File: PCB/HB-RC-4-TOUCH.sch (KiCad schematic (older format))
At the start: 13 parts, among them J1 Pad1, J2 Pad2, J3 Pad3, J4 Pad4, J5 SCL, J6 SDA, SW1 Config, U1 CC1101, U2 MPR121_Module-Touchpad, X1 Arduino_Pro_Mini

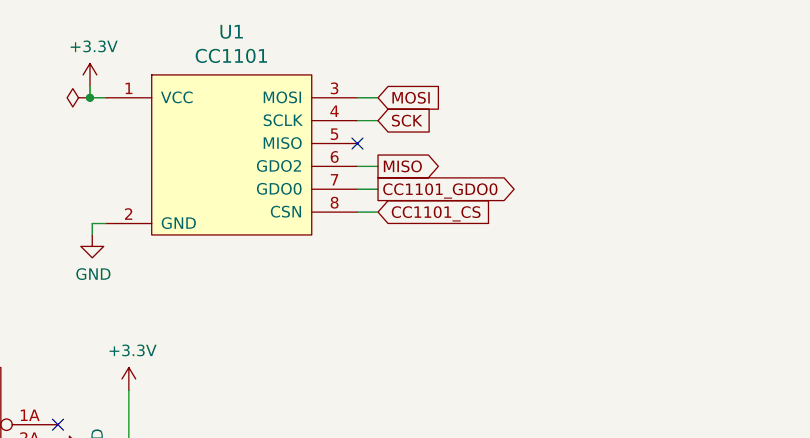
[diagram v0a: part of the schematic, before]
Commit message: update pcb
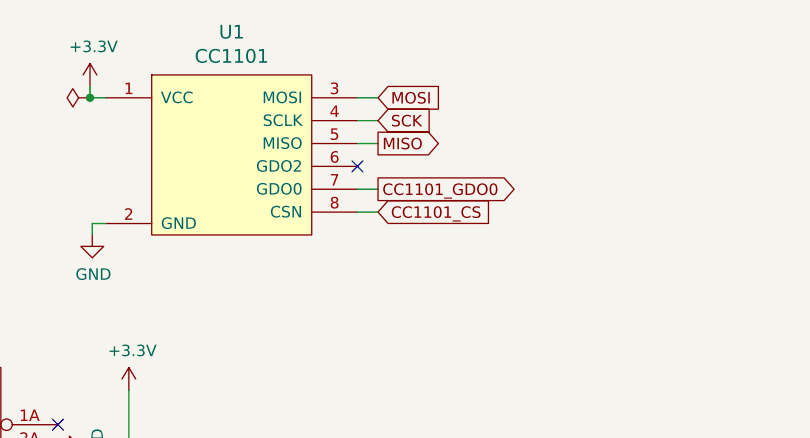
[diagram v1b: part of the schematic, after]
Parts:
- R1, R2: footprint Resistor_THT:R_Axial_DIN0207_L6.3mm_D2.5mm_P10.16mm_Horizontal -> Resistor_SMD:R_0805_2012Metric_Pad1.15x1.40mm_HandSolder
- SW1: footprint Button_Switch_SMD:SW_SPST_PTS645 -> Button_Switch_SMD:SW_SPST_FSMSM
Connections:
- net MISO: now also U1.5 (MISO); no longer U1.6 (GDO2)
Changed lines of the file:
@@
 Wire Wire Line
 	5120 1490 5210 1490
-Text GLabel 5210 1790 2    50   Output ~ 0
+Text GLabel 5210 1690 2    50   Output ~ 0
 MISO
-Wire Wire Line
-	5120 1790 5210 1790
-NoConn ~ 5120 1690
 $Comp
 L power:PWR_FLAG #FLG0101
@@
 F 0 "SW1" H 2460 4200 50  0000 C CNN
 F 1 "Config" H 2460 4280 50  0000 C CNN
-F 2 "Button_Switch_SMD:SW_SPST_PTS645" H 2460 4220 50  0001 C CNN
+F 2 "Button_Switch_SMD:SW_SPST_FSMSM" H 2460 4220 50  0001 C CNN
 F 3 "~" H 2460 4220 50  0001 C CNN
 	1    2460 4020
@@
 F 0 "R1" H 1660 4120 50  0000 L CNN
 F 1 "330" V 1790 3890 50  0000 L CNN
-F 2 "Resistor_THT:R_Axial_DIN0207_L6.3mm_D2.5mm_P10.16mm_Horizontal" V 1720 3960 50  0001 C CNN
+F 2 "Resistor_SMD:R_0805_2012Metric_Pad1.15x1.40mm_HandSolder" V 1720 3960 50  0001 C CNN
 F 3 "~" H 1790 3960 50  0001 C CNN
 	1    1790 3960
@@
 F 0 "R2" H 1870 4130 50  0000 L CNN
 F 1 "330" V 1990 3890 50  0000 L CNN
-F 2 "Resistor_THT:R_Axial_DIN0207_L6.3mm_D2.5mm_P10.16mm_Horizontal" V 1920 3960 50  0001 C CNN
+F 2 "Resistor_SMD:R_0805_2012Metric_Pad1.15x1.40mm_HandSolder" V 1920 3960 50  0001 C CNN
 F 3 "~" H 1990 3960 50  0001 C CNN
 	1    1990 3960
@@
 	-1   0    0    1
 $EndComp
+Wire Wire Line
+	5120 1690 5210 1690
+NoConn ~ 5120 1790
 $EndSCHEMATC
